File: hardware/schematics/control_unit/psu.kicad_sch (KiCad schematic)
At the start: 12 parts, among them U16 LM2596T-ADJ

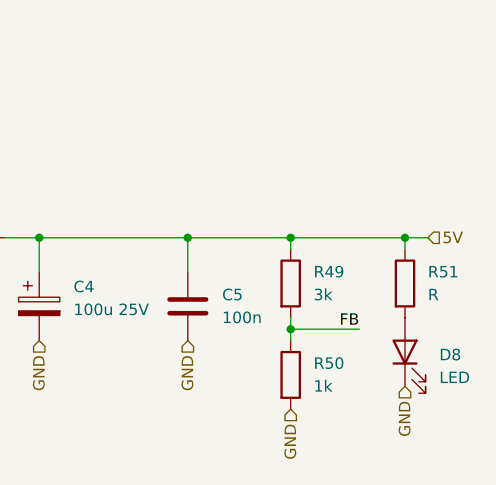
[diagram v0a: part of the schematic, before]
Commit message: !feat
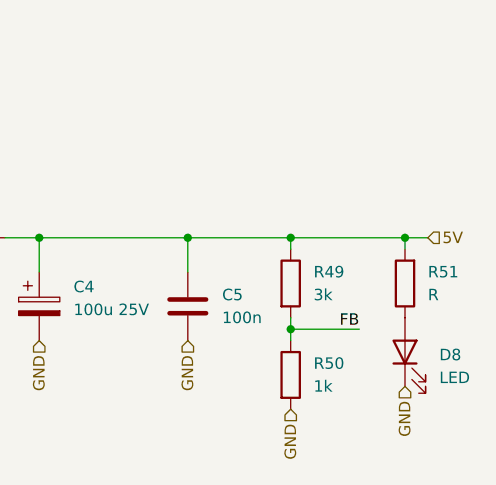
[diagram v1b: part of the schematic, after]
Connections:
- net 5V: now also R51.2; no longer R51.1
- net at D8.2 (A): now also R51.1; no longer R51.2
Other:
- moved on the sheet: R51
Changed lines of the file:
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@@
 	(symbol
 		(lib_id "Device:R")
-		(at 215.9 92.71 0)
+		(at 215.9 92.71 180)
 		(unit 1)
 		(exclude_from_sim no)
@@
 					(size 1.27 1.27)
 				)
-				(justify left)
+				(justify right)
 			)
 		)
@@
 					(size 1.27 1.27)
 				)
-				(justify left)
+				(justify right)
 			)
 		)
 		(property "Footprint" "Resistor_THT:R_Axial_DIN0207_L6.3mm_D2.5mm_P7.62mm_Horizontal"
-			(at 214.122 92.71 90)
+			(at 217.678 92.71 90)
 			(effects
 				(font
